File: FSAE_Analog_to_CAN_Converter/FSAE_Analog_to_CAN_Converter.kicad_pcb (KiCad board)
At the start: 4 copper layers, 37 parts, among them J1 Conn_01x07_Pin, J2 Conn_01x02_Pin, J3 Conn_01x05, U1 AP63205WU, U2 LT1962-3.3, U3 STM32F103RCTx, U4 MCP2561-E-MF, Y1 8MHz

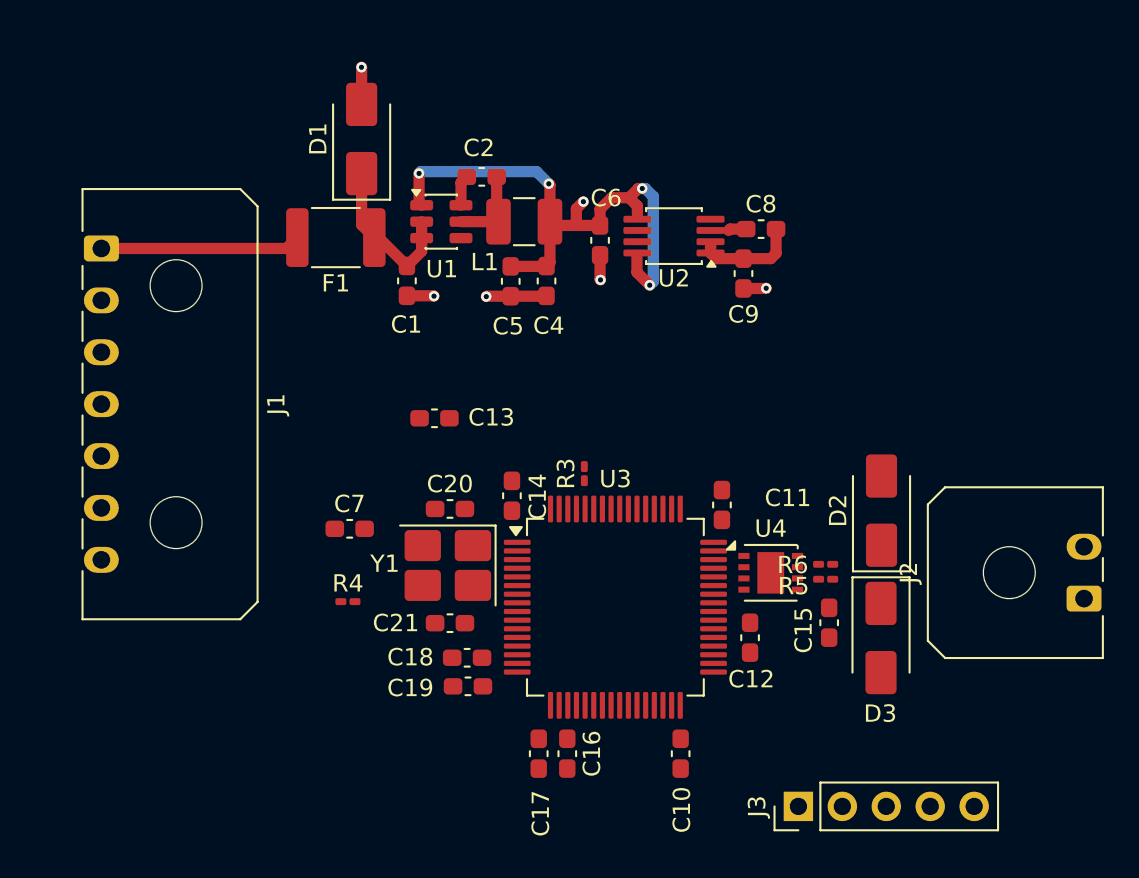
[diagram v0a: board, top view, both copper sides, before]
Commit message: almost done
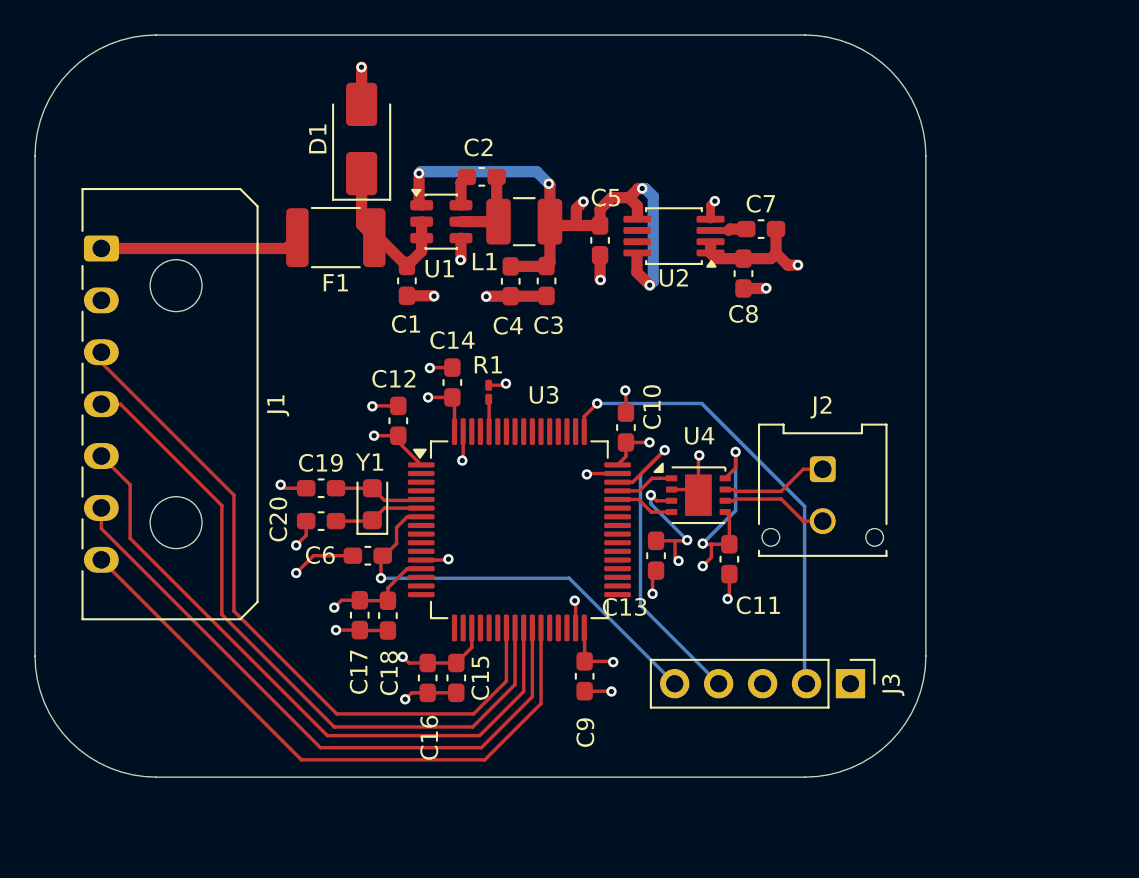
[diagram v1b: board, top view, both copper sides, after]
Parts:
- removed the C12 at (93.7, 60.7)
- removed the C15 at (98.3, 59.9)
- removed D2, D3: SMAJ16A, Diode_SMD:D_SMA
- removed R4: 10k, Resistor_SMD:R_0201_0603Metric_Pad0.64x0.40mm_HandSolder
- removed R5, R6: 60, Resistor_SMD:R_0201_0603Metric_Pad0.64x0.40mm_HandSolder
- added C11: 100nF, Capacitor_SMD:C_0603_1608Metric_Pad1.08x0.95mm_HandSolder, F.Cu at (92.5, 56.2)
- added C13: 100nF, Capacitor_SMD:C_0603_1608Metric_Pad1.08x0.95mm_HandSolder, F.Cu at (88.3, 56.0)
- J2: footprint Connector_Molex:Molex_Micro-Fit_3.0_43650-0200_1x02_P3.00mm_Horizontal -> Connector_Molex:Molex_Micro-Fit_3.0_43045-0212_2x01_P3.00mm_Vertical
- U4: value MCP2561-E-MF -> MCP2562-E-MF
- Y1: footprint Crystal:Crystal_SMD_3225-4Pin_3.2x2.5mm_HandSoldering -> Crystal:Crystal_SMD_2012-2Pin_2.0x1.2mm_HandSoldering
- moved J2 16.9 mm to (97.9, 51.0), turned to 0 degrees
- moved C20 9.51 mm to (68.9, 54.0), turned to 0 degrees
- moved C16 7.77 mm to (75.1, 63.1)
- moved C15 7.77 mm to (76.8, 63.1)
- moved J3 7.70 mm to (99.5, 63.4), turned to -90 degrees
- moved C19 7.55 mm to (68.9, 52.1)
- moved C14 7.40 mm to (76.5, 46.0)
- moved R1 7.26 mm to (78.6, 46.5)
- moved C10 7.13 mm to (86.6, 48.6)
- moved U3 7.13 mm to (80.4, 54.5)
- moved C9 7.13 mm to (84.2, 63.0)
- moved C17 6.68 mm to (71.2, 59.4), turned to -90 degrees
- moved C18 6.18 mm to (72.8, 59.5), turned to -90 degrees
- moved U4 6.13 mm to (90.8, 52.5)
- moved Y1 5.62 mm to (71.9, 53.0), turned to 90 degrees
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- renumbered C11 to C10, C13 to C12, C16 to C15, C17 to C16, C18 to C17, C19 to C18, C20 to C19, C21 to C20, C4 to C3, C5 to C4, C6 to C5, C7 to C6, C8 to C7, C9 to C8, C10 to C9, R3 to R1
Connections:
- net Net-(U3-PA11) renamed /CAN_RX
- net Net-(U3-PA12) renamed /CAN_TX
- C19 pad 2: /OSC_IN -> /OSC_P
- C20 pad 2: /OSC_OUT -> /OSC_N
- J2 pad 1: Net-(D3-A1) -> /CAN_OUT_P
- J2 pad 2: Net-(D2-A1) -> /CAN_OUT_N
- U3 pad 14: /AIN_1 -> unconnected-(U3-PA0-Pad14)
- U3 pad 15: /AIN_2 -> unconnected-(U3-PA1-Pad15)
- U3 pad 16: /AIN_3 -> unconnected-(U3-PA2-Pad16)
- U3 pad 17: /AIN_4 -> unconnected-(U3-PA3-Pad17)
- U3 pad 20: /AIN_5 -> unconnected-(U3-PA4-Pad20)
- U3 pad 23: unconnected-(U3-PA7-Pad23) -> /AIN_1
- U3 pad 24: unconnected-(U3-PC4-Pad24) -> /AIN_2
- U3 pad 25: unconnected-(U3-PC5-Pad25) -> /AIN_3
- U3 pad 26: unconnected-(U3-PB0-Pad26) -> /AIN_4
- U3 pad 27: unconnected-(U3-PB1-Pad27) -> /AIN_5
- U3 pad 41: Net-(U3-PA8) -> unconnected-(U3-PA8-Pad41)
- U3 pad 5: /OSC_IN -> /OSC_P
- U3 pad 6: /OSC_OUT -> /OSC_N
- U4 pad 5: Net-(U4-SPLIT) -> +3.3V
- U4 pad 6: Net-(D3-A1) -> /CAN_OUT_N
- U4 pad 7: Net-(D2-A1) -> /CAN_OUT_P
- U4 pad 8: Net-(U3-PA8) -> +3.3V
- Y1 pad 1: /OSC_IN -> /OSC_N
- Y1 pad 2: GND -> /OSC_P
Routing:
- net /AIN_1: track 0.00 -> 40.2 mm
- net /AIN_2: track 0.00 -> 39.6 mm
- net +3.3V: track 6.42 -> 45.8 mm, vias 0 -> 10
- net /AIN_3: track 0.00 -> 37.7 mm
- net /AIN_4: track 0.00 -> 36.6 mm
- net /AIN_5: track 0.00 -> 35.9 mm
- net GND: track 10.0 -> 45.3 mm, vias 5 -> 24
- net /SWCLK: track 0.00 -> 26.7 mm, vias 0 -> 1
- net /NRST: track 0.00 -> 24.8 mm, vias 0 -> 1
- net /SWDIO: track 0.00 -> 19.4 mm, vias 0 -> 1
- net +5V: track 34.2 -> 42.1 mm, vias 5 -> 8
- net /CAN_OUT_N: track 0.00 -> 6.21 mm
- net /CAN_OUT_P: track 0.00 -> 6.21 mm
- net /OSC_N: track 0.00 -> 5.24 mm
- net /OSC_P: track 0.00 -> 5.24 mm
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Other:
- board outline added: 51.5 x 42.9 mm

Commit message: production files and no DRC errors
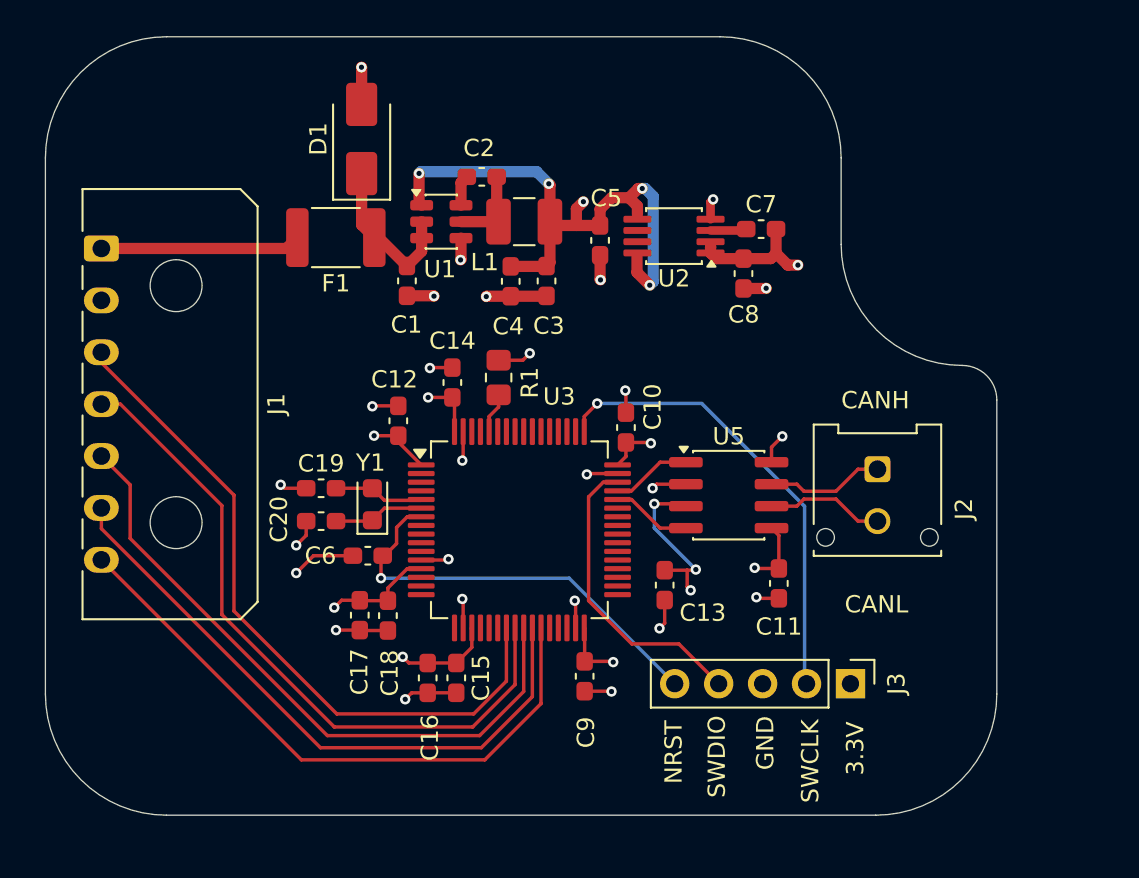
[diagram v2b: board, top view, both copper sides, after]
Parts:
- removed U4: MCP2562-E-MF, Package_DFN_QFN:DFN-8-1EP_3x3mm_P0.65mm_EP1.55x2.4mm
- added U5: MCP2562-E-SN, Package_SO:SOIC-8_3.9x4.9mm_P1.27mm, F.Cu at (92.5, 52.5)
- R1: footprint Resistor_SMD:R_0201_0603Metric_Pad0.64x0.40mm_HandSolder -> Resistor_SMD:R_0805_2012Metric_Pad1.20x1.40mm_HandSolder
- moved C11 3.19 mm to (95.4, 57.6)
- moved J2 3.16 mm to (101.1, 51.0)
- moved C13 1.77 mm to (88.8, 57.7)
- moved R1 1.03 mm to (79.2, 45.7)
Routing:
- net +3.3V: track 45.8 -> 37.0 mm, vias 10 -> 8
- net GND: track 45.3 -> 48.1 mm, vias 24 -> 26
- net /SWDIO: track 19.4 -> 17.5 mm, vias 1 -> 0
- net +5V: track 42.1 -> 44.0 mm
- net /CAN_TX: track 3.43 -> 4.64 mm
- net /CAN_RX: track 3.43 -> 4.64 mm
- net Net-(U2-BYP): track 1.05 -> 2.10 mm
- net /CAN_OUT_P: track 6.21 -> 6.82 mm
- net /CAN_OUT_N: track 6.21 -> 6.82 mm
- added copper zone on In2.Cu, net +5V
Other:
- board size 51.5 x 42.9 mm -> 55 x 45 mm
- board text added: "3.3V"
- board text added: "CANH"
- board text added: "CANL"
- board text added: "GND"
- board text added: "NRST"
- board text added: "SWCLK"
- board text added: "SWDIO"
